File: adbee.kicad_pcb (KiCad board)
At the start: 2 copper layers, 21.5 x 37 mm, 8 parts, among them J1 MD-40SM, M1 Module_XIAO-ESP32S3, Q1 BSS138

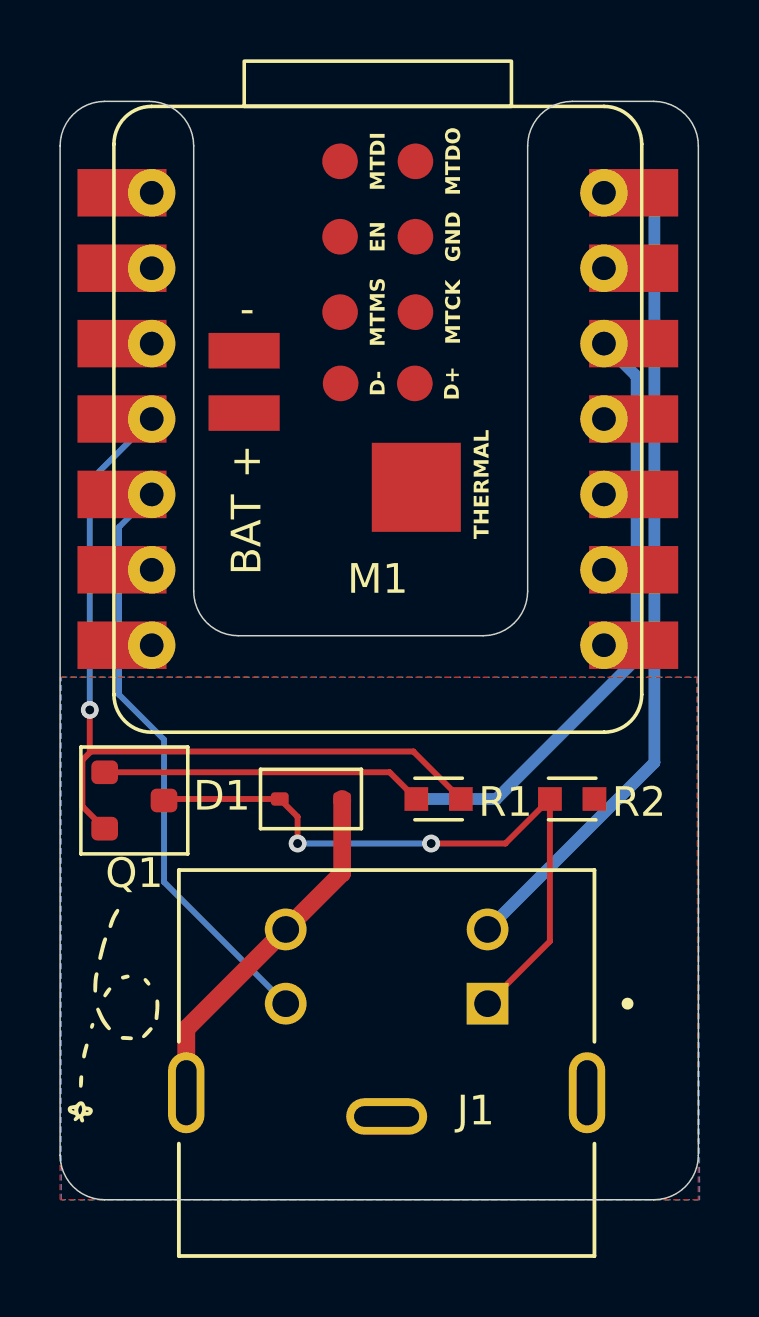
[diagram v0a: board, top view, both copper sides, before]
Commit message: finalizing
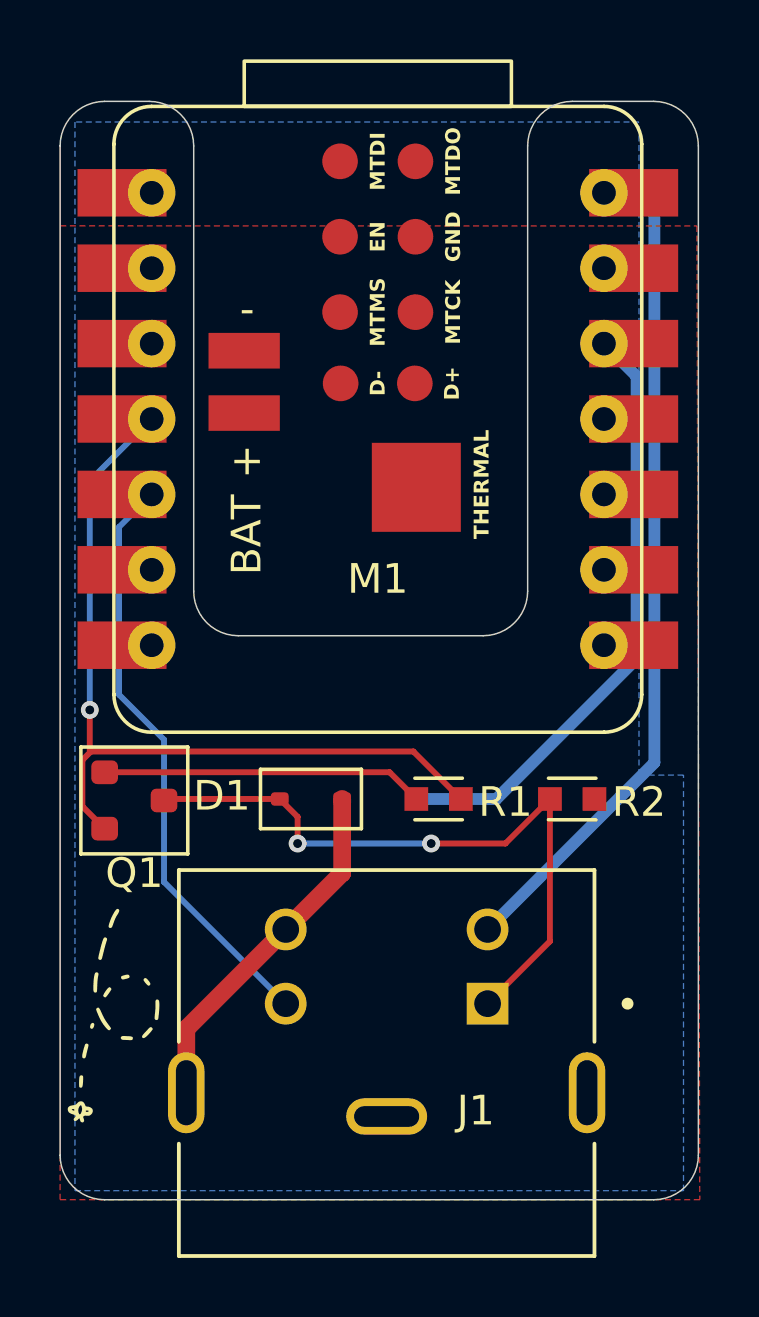
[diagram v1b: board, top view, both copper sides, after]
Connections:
- M1 pad 13: unconnected-(M1-GND-Pad13) -> GND
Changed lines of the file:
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@@
 			(outputformat 1)
 			(mirror no)
-			(drillshape 1)
+			(drillshape 0)
 			(scaleselection 1)
-			(outputdirectory "")
+			(outputdirectory "output/")
 		)
 	)
@@
 			(layers "*.Cu" "*.Mask")
 			(remove_unused_layers no)
-			(net "unconnected-(M1-GND-Pad13)_1")
+			(net "GND")
 			(pinfunction "GND_13")
-			(pintype "power_in+no_connect")
+			(pintype "power_in")
 		)
 		(pad "13" smd rect
@@
 			)
 			(layers "F.Cu" "F.Mask" "F.Paste")
-			(net "unconnected-(M1-GND-Pad13)")
+			(net "GND")
 			(pinfunction "GND_13")
-			(pintype "power_in+no_connect")
+			(pintype "power_in")
 		)
 		(pad "14" thru_hole circle
@@
 		(stroke
 			(width 0.05)
-			(type default)
+			(type solid)
 		)
 		(layer "Edge.Cuts")
@@
 		(polygon
 			(pts
-				(xy 134.003234 105.203016) (xy 155.448015 105.206957) (xy 155.5 122.805) (xy 134 122.805)
+				(xy 134.006028 89.998161) (xy 155.451265 90.002104) (xy 155.548166 122.805) (xy 134 122.805)
 			)
 		)
@@
 		(layer "B.Cu")
 		(hatch edge 0.5)
+		(priority 1)
 		(connect_pads
 			(clearance 0.5)
@@
 		(polygon
 			(pts
-				(xy 134.043271 105.203023) (xy 155.488052 105.206964) (xy 155.540037 122.805) (xy 134.040037 122.805)
-			)
-		)
+				(xy 134.5 86.5) (xy 134.5 122.5) (xy 155 122.5) (xy 155 108.5) (xy 153.5 108.5) (xy 153.5 86.5)
+			)
+		)
